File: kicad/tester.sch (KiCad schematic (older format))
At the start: 44 parts

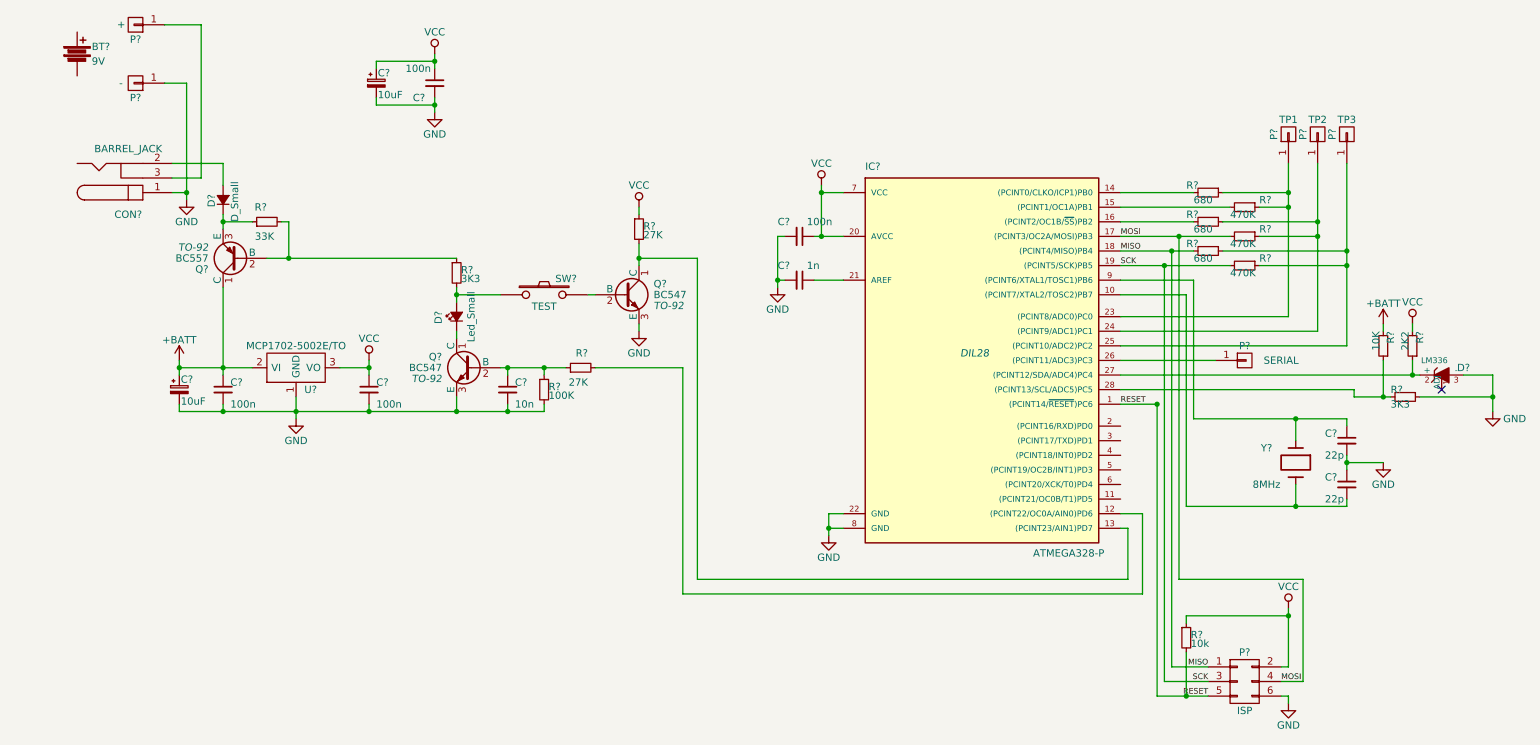
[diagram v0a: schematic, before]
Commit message: Schematic capture almost complete
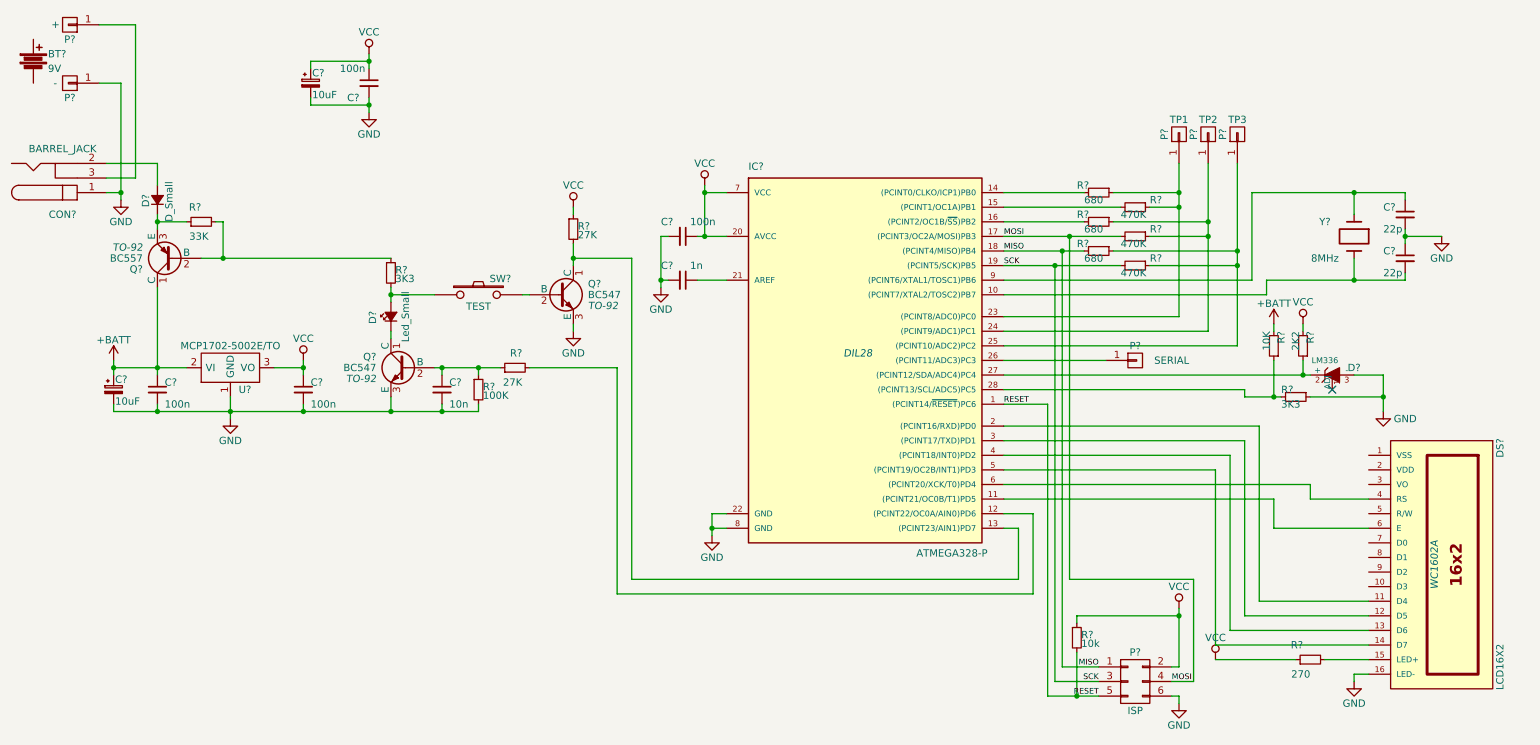
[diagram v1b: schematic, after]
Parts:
- added DS?: LCD16X2, WC1602A, symbol LCD16X2
- added R?: 270, symbol R_Small
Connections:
- net GND: now also DS?.16 (LED-)
- net VCC: now also R?.1
- net at IC?.11 ((PCINT21/OC0B/T1)PD5): now also DS?.6 (E)
- net at IC?.2 ((PCINT16/RXD)PD0): now also DS?.11 (D4)
- net at IC?.3 ((PCINT17/TXD)PD1): now also DS?.12 (D5)
- net at IC?.4 ((PCINT18/INT0)PD2): now also DS?.13 (D6)
- net at IC?.5 ((PCINT19/OC2B/INT1)PD3): now also DS?.14 (D7)
- net at IC?.6 ((PCINT20/XCK/T0)PD4): now also DS?.4 (RS)
- new net: DS?.15 (LED+), R?.2
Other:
- moved on the sheet: BT?, C?, CON?, D?, IC?, P?, Q?, R?, SW?, U?, Y?
